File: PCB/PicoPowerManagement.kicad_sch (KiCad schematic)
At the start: 25 parts, among them J1 Conn_02x07_Odd_Even, J10 Conn_02x07_Odd_Even, J11 NAS Fan 1, J12 NAS Fan 2, J13 ATX 24P Connection, J15 Conn_01x02, J2 Conn_02x07_Odd_Even, J3 UART Header, J4 DEBUG, J5 SwitchLEDS, J6 Conn_02x07_Odd_Even, J7 Conn_02x07_Odd_Even, J8 PowerSwitch, J9 Conn_02x07_Odd_Even, Q1 2N3904, SW1 SW_SPST, U2 LP5810ADSDR, U3 LP5810ADSDR, U4 LSF0101DRYR, U5 LSF0101DRYR

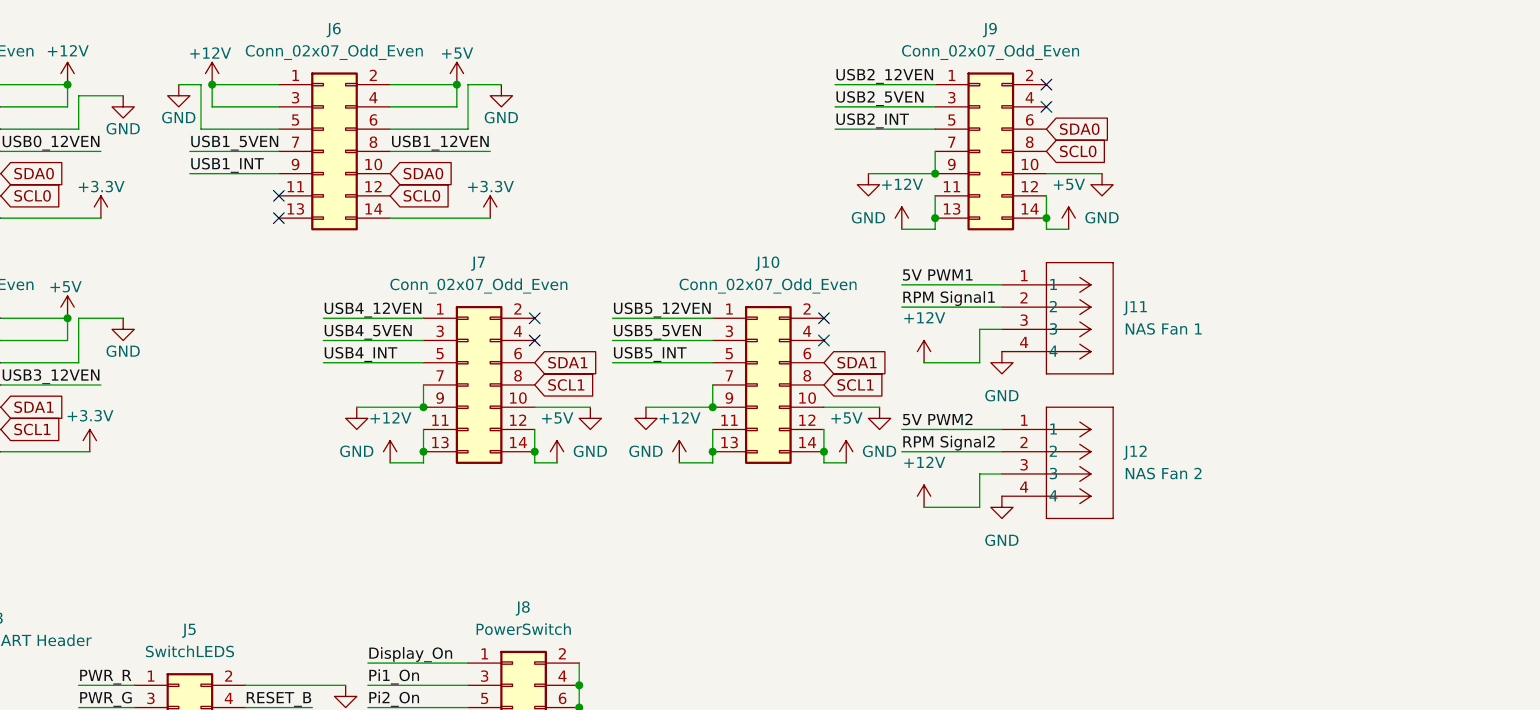
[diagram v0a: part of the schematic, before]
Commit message: confused now
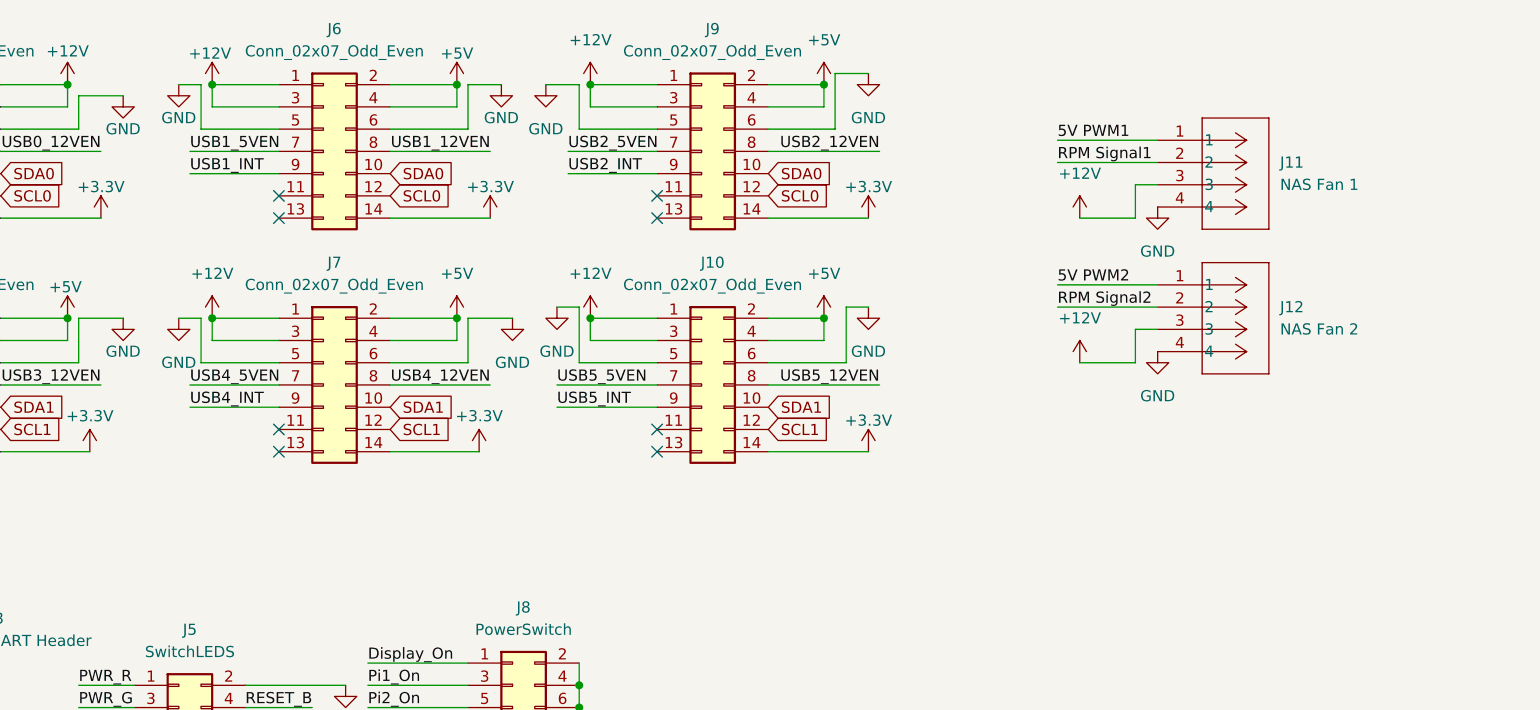
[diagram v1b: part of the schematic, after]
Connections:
- net +12V: now also J10.1 (Pin_1), J10.3 (Pin_3), J7.1 (Pin_1), J7.3 (Pin_3), J9.1 (Pin_1), J9.3 (Pin_3); no longer J10.11 (Pin_11), J10.13 (Pin_13), J7.11 (Pin_11), J7.13 (Pin_13), J9.11 (Pin_11), J9.13 (Pin_13)
- net +3.3V: now also J10.14 (Pin_14), J7.14 (Pin_14), J9.14 (Pin_14)
- net +5V: now also J10.2 (Pin_2), J10.4 (Pin_4), J7.2 (Pin_2), J7.4 (Pin_4), J9.2 (Pin_2), J9.4 (Pin_4); no longer J10.12 (Pin_12), J10.14 (Pin_14), J7.12 (Pin_12), J7.14 (Pin_14), J9.12 (Pin_12), J9.14 (Pin_14)
- net GND: now also J10.5 (Pin_5), J10.6 (Pin_6), J7.5 (Pin_5), J7.6 (Pin_6), J9.5 (Pin_5), J9.6 (Pin_6); no longer J10.10 (Pin_10), J10.7 (Pin_7), J10.9 (Pin_9), J7.10 (Pin_10), J7.7 (Pin_7), J7.9 (Pin_9), J9.10 (Pin_10), J9.7 (Pin_7), J9.9 (Pin_9)
- net SCL0: now also J9.12 (Pin_12); no longer J9.8 (Pin_8)
- net SCL1: now also J10.12 (Pin_12), J7.12 (Pin_12); no longer J10.8 (Pin_8), J7.8 (Pin_8)
- net SDA0: now also J9.10 (Pin_10); no longer J9.6 (Pin_6)
- net SDA1: now also J10.10 (Pin_10), J7.10 (Pin_10); no longer J10.6 (Pin_6), J7.6 (Pin_6)
- net USB2_12VEN: now also J9.8 (Pin_8); no longer J9.1 (Pin_1)
- net USB2_5VEN: now also J9.7 (Pin_7); no longer J9.3 (Pin_3)
- net USB2_INT: now also J9.9 (Pin_9); no longer J9.5 (Pin_5)
- net USB4_12VEN: now also J7.8 (Pin_8); no longer J7.1 (Pin_1)
- net USB4_5VEN: now also J7.7 (Pin_7); no longer J7.3 (Pin_3)
- net USB4_INT: now also J7.9 (Pin_9); no longer J7.5 (Pin_5)
- net USB5_12VEN: now also J10.8 (Pin_8); no longer J10.1 (Pin_1)
- net USB5_5VEN: now also J10.7 (Pin_7); no longer J10.3 (Pin_3)
- net USB5_INT: now also J10.9 (Pin_9); no longer J10.5 (Pin_5)
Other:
- moved on the sheet: J10, J11, J12, J7, J9
